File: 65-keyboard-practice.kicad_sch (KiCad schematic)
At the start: 2 parts, among them SW1 SW_MEC_5E, U1 ProMicro

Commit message: half wiring done
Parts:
- SW1: footprint (none) -> random-keyboard-parts:PushButton_6x6mm_TH
- U1: footprint (none) -> Keebio-Parts:ArduinoProMicro

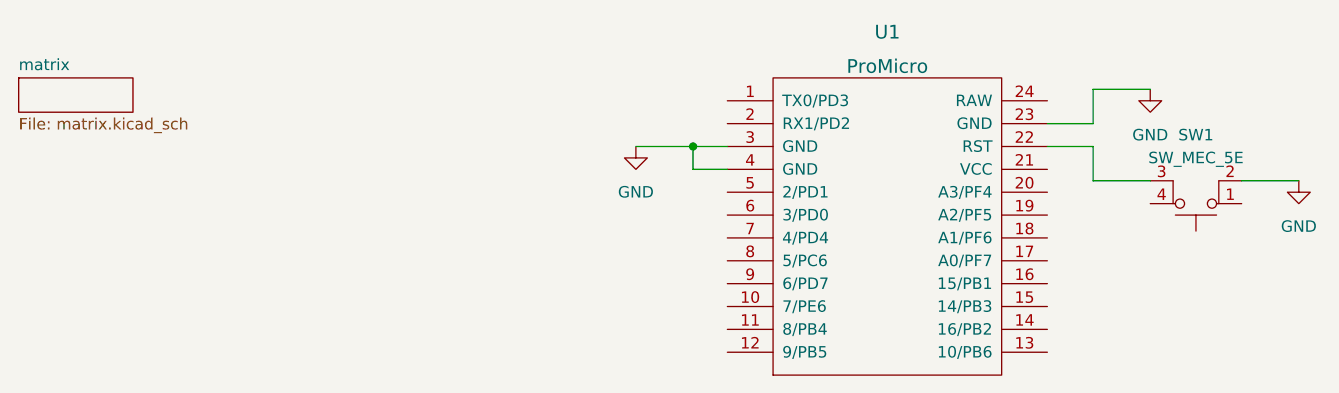
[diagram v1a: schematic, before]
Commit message: Finished the design
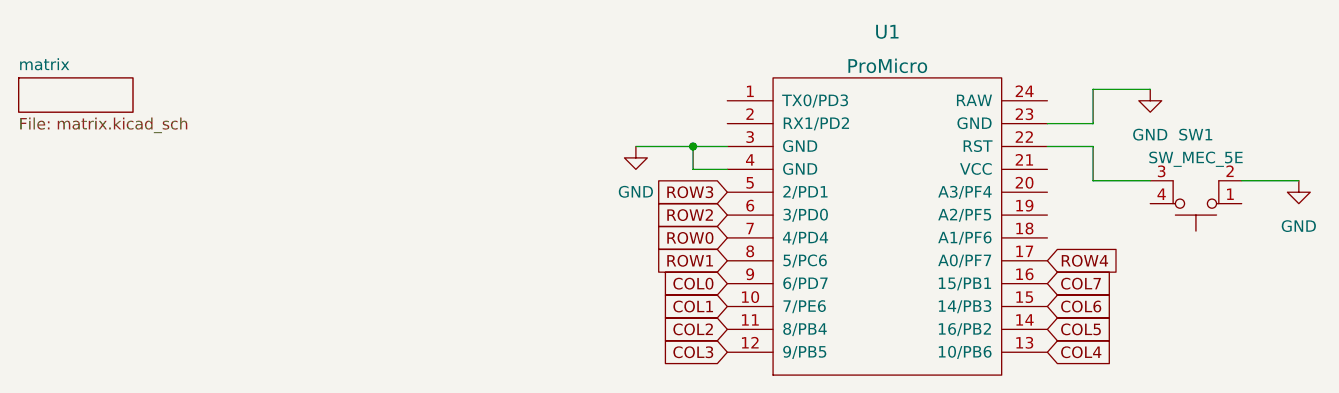
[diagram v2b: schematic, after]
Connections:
- net COL1: now reaches U1.10 (7/PE6)
- net COL2: now reaches U1.11 (8/PB4)
- net COL3: now reaches U1.12 (9/PB5)
- net COL4: now reaches U1.13 (10/PB6)
- net COL5: now reaches U1.14 (16/PB2)
- net COL6: now reaches U1.15 (14/PB3)
- net COL7: now reaches U1.16 (15/PB1)
- net ROW4: now reaches U1.17 (A0/PF7)
- net ROW3: now reaches U1.5 (2/PD1)
- net ROW2: now reaches U1.6 (3/PD0)
- net ROW0: now reaches U1.7 (4/PD4)
- net ROW1: now reaches U1.8 (5/PC6)
- net COL0: now reaches U1.9 (6/PD7)
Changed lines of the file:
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@@
     (stroke (width 0) (type default) (color 0 0 0 0))
+  )
+  (global_label "ROW1" (shape input) (at 214.63 71.12 180) (fields_autoplaced)
+    (effects (font (size 1.27 1.27)) (justify right))
+    (property "Intersheet References" "${INTERSHEET_REFS}" (id 0) (at 206.9555 71.0406 0)
+      (effects (font (size 1.27 1.27)) (justify right) hide)
+    )
+  )
+  (global_label "ROW4" (shape input) (at 250.19 71.12 0) (fields_autoplaced)
+    (effects (font (size 1.27 1.27)) (justify left))
+    (property "Intersheet References" "${INTERSHEET_REFS}" (id 0) (at 257.8645 71.0406 0)
+      (effects (font (size 1.27 1.27)) (justify left) hide)
+    )
+  )
+  (global_label "COL0" (shape input) (at 214.63 73.66 180) (fields_autoplaced)
+    (effects (font (size 1.27 1.27)) (justify right))
+    (property "Intersheet References" "${INTERSHEET_REFS}" (id 0) (at 207.3788 73.5806 0)
+      (effects (font (size 1.27 1.27)) (justify right) hide)
+    )
+  )
+  (global_label "COL2" (shape input) (at 214.63 78.74 180) (fields_autoplaced)
+    (effects (font (size 1.27 1.27)) (justify right))
+    (property "Intersheet References" "${INTERSHEET_REFS}" (id 0) (at 207.3788 78.6606 0)
+      (effects (font (size 1.27 1.27)) (justify right) hide)
+    )
+  )
+  (global_label "ROW0" (shape input) (at 214.63 68.58 180) (fields_autoplaced)
+    (effects (font (size 1.27 1.27)) (justify right))
+    (property "Intersheet References" "${INTERSHEET_REFS}" (id 0) (at 206.9555 68.5006 0)
+      (effects (font (size 1.27 1.27)) (justify right) hide)
+    )
+  )
+  (global_label "COL3" (shape input) (at 214.63 81.28 180) (fields_autoplaced)
+    (effects (font (size 1.27 1.27)) (justify right))
+    (property "Intersheet References" "${INTERSHEET_REFS}" (id 0) (at 207.3788 81.2006 0)
+      (effects (font (size 1.27 1.27)) (justify right) hide)
+    )
+  )
+  (global_label "COL1" (shape input) (at 214.63 76.2 180) (fields_autoplaced)
+    (effects (font (size 1.27 1.27)) (justify right))
+    (property "Intersheet References" "${INTERSHEET_REFS}" (id 0) (at 207.3788 76.1206 0)
+      (effects (font (size 1.27 1.27)) (justify right) hide)
+    )
+  )
+  (global_label "COL4" (shape input) (at 250.19 81.28 0) (fields_autoplaced)
+    (effects (font (size 1.27 1.27)) (justify left))
+    (property "Intersheet References" "${INTERSHEET_REFS}" (id 0) (at 257.4412 81.2006 0)
+      (effects (font (size 1.27 1.27)) (justify left) hide)
+    )
+  )
+  (global_label "ROW3" (shape input) (at 214.63 63.5 180) (fields_autoplaced)
+    (effects (font (size 1.27 1.27)) (justify right))
+    (property "Intersheet References" "${INTERSHEET_REFS}" (id 0) (at 206.9555 63.4206 0)
+      (effects (font (size 1.27 1.27)) (justify right) hide)
+    )
+  )
+  (global_label "COL5" (shape input) (at 250.19 78.74 0) (fields_autoplaced)
+    (effects (font (size 1.27 1.27)) (justify left))
+    (property "Intersheet References" "${INTERSHEET_REFS}" (id 0) (at 257.4412 78.6606 0)
+      (effects (font (size 1.27 1.27)) (justify left) hide)
+    )
+  )
+  (global_label "COL7" (shape input) (at 250.19 73.66 0) (fields_autoplaced)
+    (effects (font (size 1.27 1.27)) (justify left))
+    (property "Intersheet References" "${INTERSHEET_REFS}" (id 0) (at 257.4412 73.5806 0)
+      (effects (font (size 1.27 1.27)) (justify left) hide)
+    )
+  )
+  (global_label "ROW2" (shape input) (at 214.63 66.04 180) (fields_autoplaced)
+    (effects (font (size 1.27 1.27)) (justify right))
+    (property "Intersheet References" "${INTERSHEET_REFS}" (id 0) (at 206.9555 65.9606 0)
+      (effects (font (size 1.27 1.27)) (justify right) hide)
+    )
+  )
+  (global_label "COL6" (shape input) (at 250.19 76.2 0) (fields_autoplaced)
+    (effects (font (size 1.27 1.27)) (justify left))
+    (property "Intersheet References" "${INTERSHEET_REFS}" (id 0) (at 257.4412 76.1206 0)
+      (effects (font (size 1.27 1.27)) (justify left) hide)
+    )
   )
   (symbol (lib_id "power:GND") (at 204.47 58.42 0) (unit 1)
